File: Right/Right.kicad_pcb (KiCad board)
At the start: 2 copper layers, 316.7 x 290.8 mm, 226 parts, among them SW0 SW_PUSH, SW1 SW_PUSH, SW10 SW_PUSH, SW100 SW_PUSH, SW1000 SW_Push_Dual_R, SW1001 SW_Push_Dual_R, SW1002 SW_Push_Dual_R, SW1003 SW_Push_Dual_R, SW1004 SW_Push_Dual_R, SW1005 SW_Push_Dual_R, SW101 SW_PUSH, SW102 SW_PUSH, SW103 SW_PUSH, SW104 SW_PUSH, SW105 SW_PUSH, SW106 SW_PUSH, SW11 SW_PUSH, SW110 SW_PUSH, SW111 SW_PUSH, SW112 SW_PUSH, SW113 SW_PUSH, SW114 SW_PUSH, SW115 SW_PUSH, SW116 SW_PUSH, SW12 SW_PUSH, SW13 SW_PUSH, SW14 SW_PUSH, SW15 SW_PUSH, SW2 SW_PUSH, SW20 SW_PUSH, SW21 SW_PUSH, SW22 SW_PUSH, SW23 SW_PUSH, SW24 SW_PUSH, SW25 SW_PUSH, SW3 SW_PUSH, SW30 SW_PUSH, SW31 SW_PUSH, SW32 SW_PUSH, SW33 SW_PUSH, SW34 SW_PUSH, SW35 SW_PUSH, SW4 SW_PUSH, SW40 SW_PUSH, SW41 SW_PUSH, SW42 SW_PUSH, SW43 SW_PUSH, SW44 SW_PUSH, SW45 SW_PUSH, SW5 SW_PUSH, SW50 SW_PUSH, SW51 SW_PUSH, SW52 SW_PUSH, SW53 SW_PUSH, SW54 SW_PUSH, SW60 SW_PUSH, SW61 SW_PUSH, SW62 SW_PUSH, SW63 SW_PUSH, SW64 SW_PUSH, SW65 SW_PUSH, SW66 SW_PUSH, SW70 SW_PUSH, SW71 SW_PUSH, SW72 SW_PUSH, SW73 SW_PUSH, SW74 SW_PUSH, SW75 SW_PUSH, SW76 SW_PUSH, SW77 SW_PUSH, SW80 SW_PUSH, SW81 SW_PUSH, SW82 SW_PUSH, SW83 SW_PUSH, SW84 SW_PUSH, SW85 SW_PUSH, SW86 SW_PUSH, SW87 SW_PUSH, SW90 SW_PUSH, SW91 SW_PUSH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

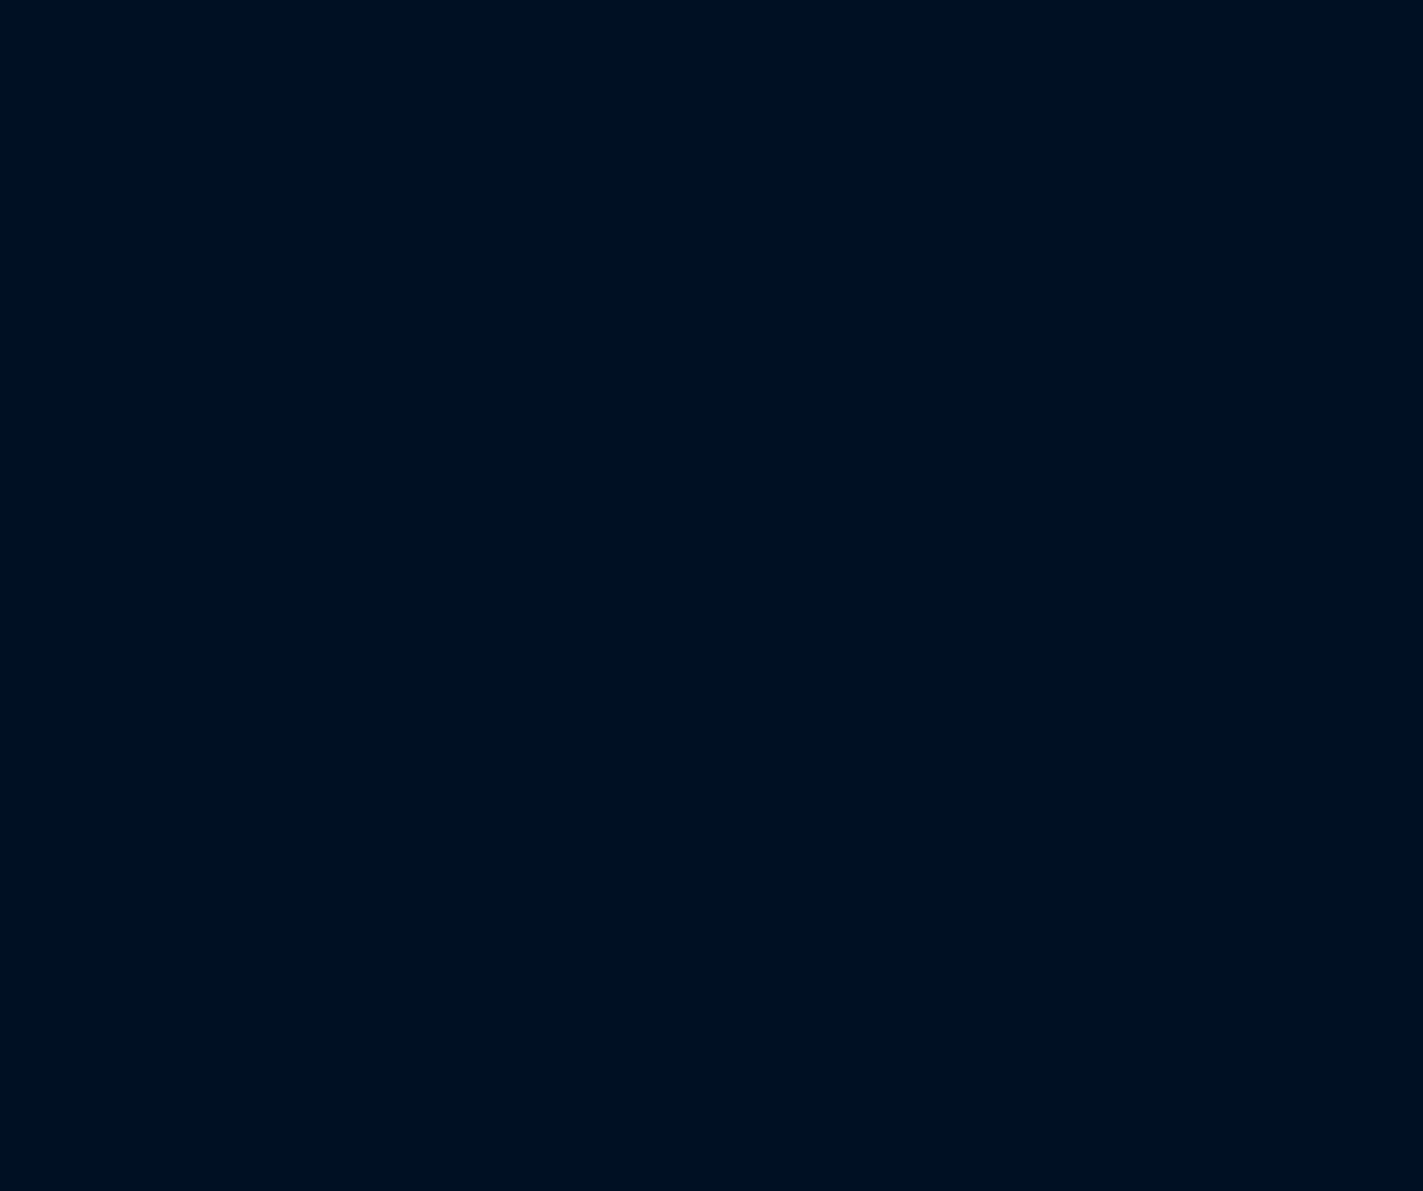
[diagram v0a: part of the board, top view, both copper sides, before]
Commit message: トッププレート
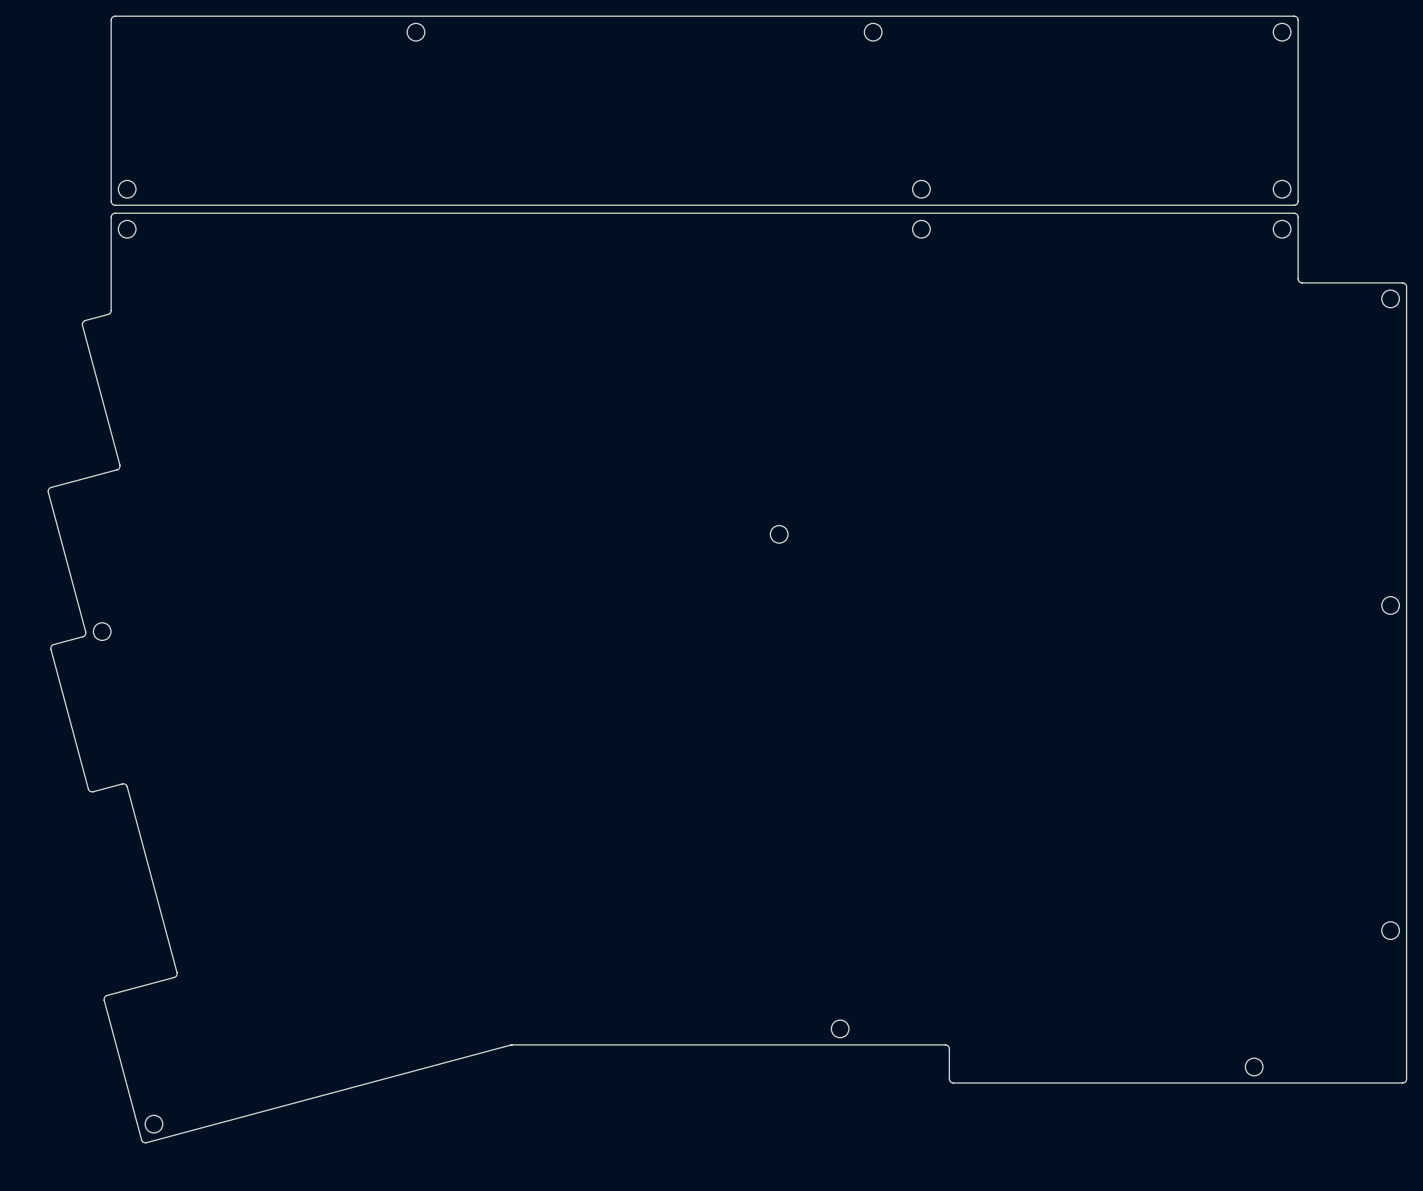
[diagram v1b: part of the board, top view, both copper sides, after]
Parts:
- added REF**: Spacer, mylibrary:Spacer, F.Cu at (159.2, -132.9)
- added REF**: Spacer, mylibrary:Spacer, F.Cu at (162.5, -21.0)
- added REF**: Spacer, mylibrary:Spacer, F.Cu at (159.2, -137.9)
- added REF**: Spacer, mylibrary:Spacer, F.Cu at (300.0, -28.2)
- added REF**: Spacer, mylibrary:Spacer, F.Cu at (317.1, -85.9)
- added REF**: Spacer, mylibrary:Spacer, F.Cu at (156.0, -82.6)
- added REF**: Spacer, mylibrary:Spacer, F.Cu at (317.1, -45.2)
- added REF**: Spacer, mylibrary:Spacer, F.Cu at (317.1, -124.2)
- added REF**: Spacer, mylibrary:Spacer, F.Cu at (252.4, -157.5)
- added REF**: Spacer, mylibrary:Spacer, F.Cu at (240.7, -94.8)
- added REF**: Spacer, mylibrary:Spacer, F.Cu at (303.5, -157.5)
- added REF**: Spacer, mylibrary:Spacer, F.Cu at (258.4, -132.9)
- added REF**: Spacer, mylibrary:Spacer, F.Cu at (248.3, -32.9)
- added REF**: Spacer, mylibrary:Spacer, F.Cu at (303.5, -137.9)
- added REF**: Spacer, mylibrary:Spacer, F.Cu at (303.5, -132.9)
- added REF**: Spacer, mylibrary:Spacer, F.Cu at (195.3, -157.5)
- added REF**: Spacer, mylibrary:Spacer, F.Cu at (258.4, -137.9)
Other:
- board size 316.7 x 290.8 mm -> 316.7 x 440.8 mm
